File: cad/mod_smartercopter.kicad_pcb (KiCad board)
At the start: 2 copper layers, 37.7 x 16.8 mm, 74 parts, among them P1 CONN_5, P2 CONN_01X01, P3 CONN_01X01, P4 CONN_2, P5 CONN_01X01, P6 CONN_01X01, P7 CONN_01X01, Q1 SiA910EDJ, SW1 SW_PUSH_4, U1 CC2541, U2 MPU-9250, U3 TPS73001, U4 TPS73001, U5 DRV8837, X1 32Mhz

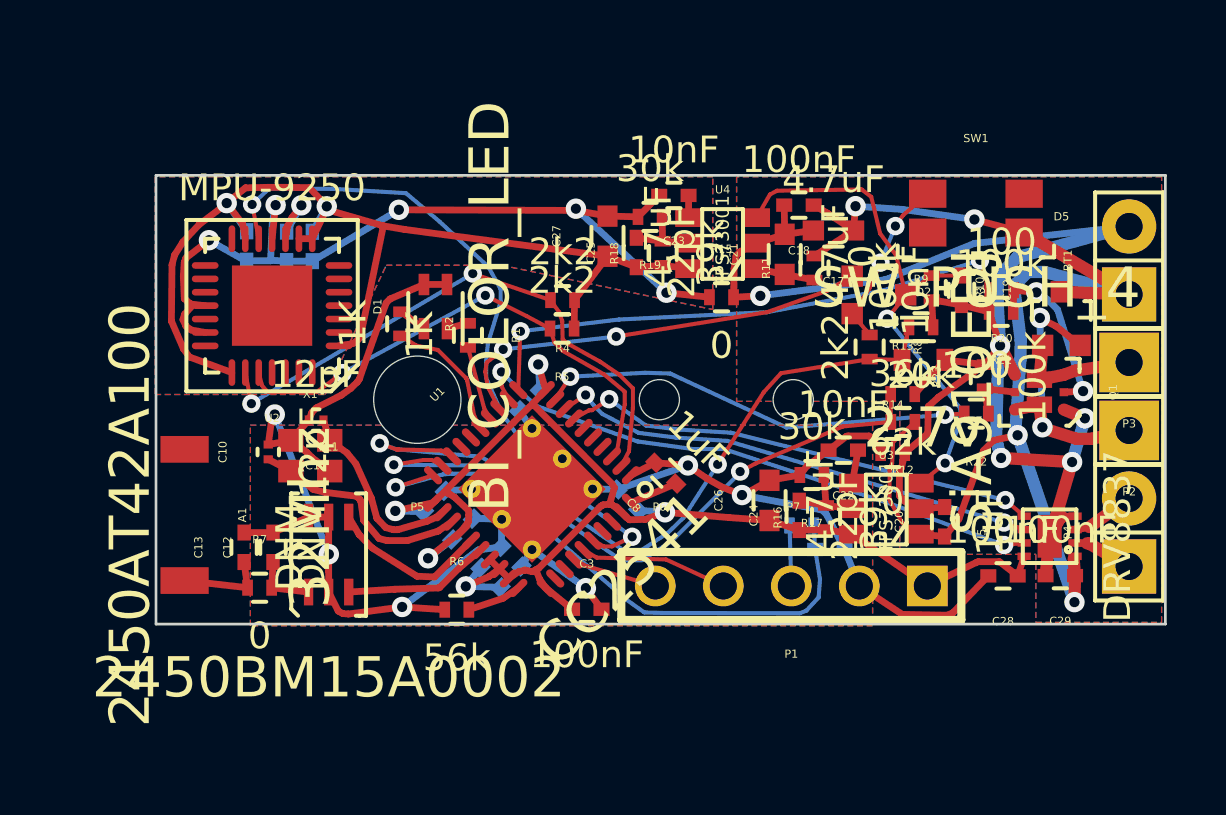
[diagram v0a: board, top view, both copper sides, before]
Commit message: moved references around
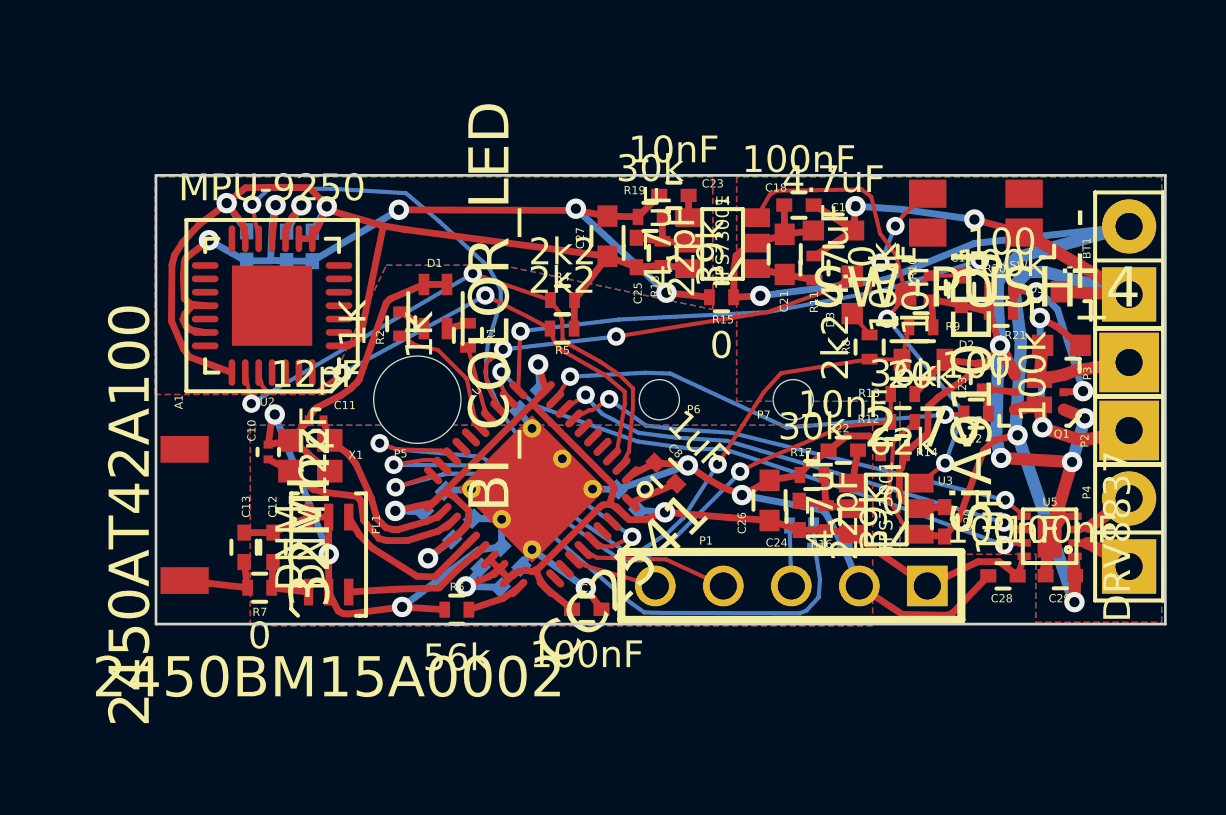
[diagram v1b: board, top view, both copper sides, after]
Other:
- board text added: "+"
- board text added: "-"
